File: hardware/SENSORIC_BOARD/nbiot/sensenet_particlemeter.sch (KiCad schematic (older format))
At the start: 102 parts, among them J1 CONN_01X01, J11 CONN_01X01, J13 BARREL_JACK, J18 CONN_01X01, J19 CONN_01X01, J2 CONN_01X01, J21 CONN_01X01, J3 CONN_01X01, J4 CONN_01X01, J5 CONN_01X01, J6 CONN_01X01, P1 SMA_mini, P2 SMA_mini, P3 CONN_02X12, Q1 Q_NMOS_GSD, SW1 SW_DPST, SW2 SW_DIP_x03, SW3 SW_DPST, U1 MC33063, U10 bme280_barebone, U2 stm32f072, U3 QUECTEL_BC95, U4 SIM, U5 CAT24C02, U6 MC33063, U7 M10578-A2, U8 usb_femalee, U9 OLED_128x64

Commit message: snazim se rozchodit novou serii, jebne me z toho z chvili
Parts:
- added C24: 2.2u, SNPM:SMD_0805, symbol C
- added J10, J12, J14, J15, J7, J8, J9: CONN_01X01, SNPM:smd_point_bottom, symbol Conn_01x01
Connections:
- wire segments 392 -> 411
- no-connect marks 87 -> 86
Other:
- note added: "PMEG4010EH,115"
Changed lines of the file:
@@
 	1    0    0    -1
 $EndComp
-NoConn ~ 9750 8800
 NoConn ~ 10050 8800
 NoConn ~ 10150 8800
@@
 	21050 7900 21150 7900
 Wire Wire Line
-	9550 8800 9550 9800
-Wire Wire Line
-	9650 8800 9650 9800
-Wire Wire Line
 	9850 9200 9850 8800
-Wire Wire Line
-	9550 9800 10100 9800
 Wire Wire Line
 	9850 9500 9850 10000
@@
 	1    0    0    -1
 $EndComp
+Wire Wire Line
+	9200 9800 9200 8950
+Wire Wire Line
+	9200 8950 9550 8950
+Wire Wire Line
+	9550 8950 9550 8800
+Wire Wire Line
+	9650 9700 9300 9700
+Wire Wire Line
+	9300 9700 9300 9050
+Wire Wire Line
+	9300 9050 9650 9050
+Wire Wire Line
+	9650 9700 9650 9800
+Wire Wire Line
+	9200 9800 10100 9800
+Wire Wire Line
+	9650 9050 9650 8800
+$Comp
+L C C24
+U 1 1 5BD086E0
+P 9600 9350
+F 0 "C24" H 9625 9450 50  0000 L CNN
+F 1 "2.2u" H 9625 9250 50  0000 L CNN
+F 2 "SNPM:SMD_0805" H 9638 9200 50  0001 C CNN
+F 3 "" H 9600 9350 50  0001 C CNN
+	1    9600 9350
+	1    0    0    -1
+$EndComp
+Wire Wire Line
+	9600 9200 9600 9150
+Wire Wire Line
+	9600 9150 9750 9150
+Wire Wire Line
+	9750 9150 9750 8800
+Wire Wire Line
+	9600 9500 9600 9600
+Wire Wire Line
+	9600 9600 9750 9600
+Wire Wire Line
+	9750 9600 9750 9800
+Connection ~ 9750 9800
+$Comp
+L Conn_01x01 J7
+U 1 1 5BD0A84C
+P 9700 10800
+F 0 "J7" V 9700 10700 50  0000 C CNN
+F 1 "CONN_01X01" V 9800 10800 50  0001 C CNN
+F 2 "SNPM:smd_point_bottom" H 9700 10800 50  0001 C CNN
+F 3 "" H 9700 10800 50  0001 C CNN
+	1    9700 10800
+	0    -1   -1   0
+$EndComp
+$Comp
+L Conn_01x01 J8
+U 1 1 5BD0BD5A
+P 9950 10800
+F 0 "J8" V 9950 10700 50  0000 C CNN
+F 1 "CONN_01X01" V 10050 10800 50  0001 C CNN
+F 2 "SNPM:smd_point_bottom" H 9950 10800 50  0001 C CNN
+F 3 "" H 9950 10800 50  0001 C CNN
+	1    9950 10800
+	0    -1   -1   0
+$EndComp
+$Comp
+L Conn_01x01 J9
+U 1 1 5BD0BEAB
+P 10200 10800
+F 0 "J9" V 10200 10700 50  0000 C CNN
+F 1 "CONN_01X01" V 10300 10800 50  0001 C CNN
+F 2 "SNPM:smd_point_bottom" H 10200 10800 50  0001 C CNN
+F 3 "" H 10200 10800 50  0001 C CNN
+	1    10200 10800
+	0    -1   -1   0
+$EndComp
+$Comp
+L Conn_01x01 J10
+U 1 1 5BD0BFFF
+P 10450 10800
+F 0 "J10" V 10450 10700 50  0000 C CNN
+F 1 "CONN_01X01" V 10550 10800 50  0001 C CNN
+F 2 "SNPM:smd_point_bottom" H 10450 10800 50  0001 C CNN
+F 3 "" H 10450 10800 50  0001 C CNN
+	1    10450 10800
+	0    -1   -1   0
+$EndComp
+$Comp
+L Conn_01x01 J12
+U 1 1 5BD0C156
+P 10700 10800
+F 0 "J12" V 10700 10700 50  0000 C CNN
+F 1 "CONN_01X01" V 10800 10800 50  0001 C CNN
+F 2 "SNPM:smd_point_bottom" H 10700 10800 50  0001 C CNN
+F 3 "" H 10700 10800 50  0001 C CNN
+	1    10700 10800
+	0    -1   -1   0
+$EndComp
+$Comp
+L Conn_01x01 J14
+U 1 1 5BD0C2BC
+P 10950 10800
+F 0 "J14" V 10950 10700 50  0000 C CNN
+F 1 "CONN_01X01" V 11050 10800 50  0001 C CNN
+F 2 "SNPM:smd_point_bottom" H 10950 10800 50  0001 C CNN
+F 3 "" H 10950 10800 50  0001 C CNN
+	1    10950 10800
+	0    -1   -1   0
+$EndComp
+$Comp
+L Conn_01x01 J15
+U 1 1 5BD0C419
+P 11200 10800
+F 0 "J15" V 11200 10700 50  0000 C CNN
+F 1 "CONN_01X01" V 11300 10800 50  0001 C CNN
+F 2 "SNPM:smd_point_bottom" H 11200 10800 50  0001 C CNN
+F 3 "" H 11200 10800 50  0001 C CNN
+	1    11200 10800
+	0    -1   -1   0
+$EndComp
+$Comp
+L GND #PWR093
+U 1 1 5BD0C6C7
+P 11200 11150
+F 0 "#PWR093" H 11200 10900 50  0001 C CNN
+F 1 "GND" H 11200 11000 50  0000 C CNN
+F 2 "" H 11200 11150 50  0001 C CNN
+F 3 "" H 11200 11150 50  0001 C CNN
+	1    11200 11150
+	1    0    0    -1
+$EndComp
+$Comp
+L +5V #PWR094
+U 1 1 5BD0D1A9
+P 10950 11150
+F 0 "#PWR094" H 10950 11000 50  0001 C CNN
+F 1 "+5V" H 10950 11290 50  0000 C CNN
+F 2 "" H 10950 11150 50  0001 C CNN
+F 3 "" H 10950 11150 50  0001 C CNN
+	1    10950 11150
+	-1   0    0    1
+$EndComp
+Text GLabel 10700 11150 3    39   Input ~ 0
+PM_SCK
+Text GLabel 10450 11150 3    39   Input ~ 0
+PM_SDO
+Text GLabel 10200 11150 3    39   Input ~ 0
+OLED_RESET
+Text GLabel 9950 11150 3    39   Input ~ 0
+OLED_D/C
+Text GLabel 9700 11150 3    39   Input ~ 0
+OLED_CS
+Wire Wire Line
+	9700 11000 9700 11150
+Wire Wire Line
+	9950 11000 9950 11150
+Wire Wire Line
+	10200 11000 10200 11150
+Wire Wire Line
+	10450 11000 10450 11150
+Wire Wire Line
+	10700 11000 10700 11150
+Wire Wire Line
+	10950 11000 10950 11150
+Wire Wire Line
+	11200 11000 11200 11150
+Text Notes 14800 1000 0    60   ~ 0
+PMEG4010EH,115
 $EndSCHEMATC

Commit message: zonglovani s repama
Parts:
- C1, C10, C11, C13, C14, C15, C16, C2, C20, C21, C22, C23, C24, C25, C3, C4, C5, C6, C7, C8, C9: symbol C -> sensenet_particlemeter-rescue:C
- C12: value 510pF -> 330pF; symbol C -> sensenet_particlemeter-rescue:C
- C17, C18, C19: symbol CP -> sensenet_particlemeter-rescue:CP
- D1, D11, D3, D5, D6: symbol D_Schottky -> sensenet_particlemeter-rescue:D_Schottky
- D10, D2, D4, D7, D8, D9: symbol LED -> sensenet_particlemeter-rescue:LED
- J1, J10, J11, J12, J14, J15, J18, J19, J2, J21, J3, J4, J5, J6, J7, J8, J9: symbol Conn_01x01 -> sensenet_particlemeter-rescue:Conn_01x01
- J13: symbol Barrel_Jack -> sensenet_particlemeter-rescue:Barrel_Jack
- L1, L2, L3, L5: symbol L -> sensenet_particlemeter-rescue:L
- L4, L6, L7, L8: symbol Ferrite_Bead -> sensenet_particlemeter-rescue:Ferrite_Bead
- LOGO1: symbol LOGO -> sensenet_particlemeter-rescue:LOGO
- P1, P2: symbol SMA_mini -> sensenet_particlemeter-rescue:SMA_mini
- P3: symbol CONN_02X12 -> sensenet_particlemeter-rescue:CONN_02X12
- Q1: symbol Q_NMOS_GSD -> sensenet_particlemeter-rescue:Q_NMOS_GSD
- R1, R10, R11, R12, R13, R14, R17, R18, R19, R2, R20, R22, R23, R24, R25, R26, R27, R28, R29, R3, R4, R5, R6, R7, R8, R9: symbol R -> sensenet_particlemeter-rescue:R
- R15: value 27k -> 2k7; symbol R -> sensenet_particlemeter-rescue:R
- R16: value 10k -> 820R; symbol R -> sensenet_particlemeter-rescue:R
- R21: value tbd -> 100R; symbol R -> sensenet_particlemeter-rescue:R
- SJ16: symbol solder_jumper -> sensenet_particlemeter-rescue:solder_jumper
- SW1, SW3: symbol SW_DPST -> sensenet_particlemeter-rescue:SW_DPST
- SW2: symbol SW_DIP_x03 -> sensenet_particlemeter-rescue:SW_DIP_x03
- U1, U6: symbol MC33063 -> sensenet_particlemeter-rescue:MC33063
- U10: symbol bme280_barebone -> sensenet_particlemeter-rescue:bme280_barebone
- U2: symbol stm32f072 -> sensenet_particlemeter-rescue:stm32f072
- U3: symbol QUECTEL_BC95 -> sensenet_particlemeter-rescue:QUECTEL_BC95
- U4: symbol SIM -> sensenet_particlemeter-rescue:SIM
- U5: symbol CAT24C02 -> sensenet_particlemeter-rescue:CAT24C02
- U7: symbol M10578-A2 -> sensenet_particlemeter-rescue:M10578-A2
- U8: symbol usb_femalee -> sensenet_particlemeter-rescue:usb_femalee
- U9: symbol OLED_128x64 -> sensenet_particlemeter-rescue:OLED_128x64
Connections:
- wire segments 411 -> 498

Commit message: rozdelane upravicky
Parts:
- removed C17: 1000u, SNPM:C_Radial_D10_L16_P5_bottom, symbol sensenet_particlemeter-rescue:CP
- removed J13: BARREL_JACK, SNPM:BARREL_JACK, symbol sensenet_particlemeter-rescue:Barrel_Jack
- added C17: 100n, Capacitor_SMD:C_0805_2012Metric, symbol sensenet_particlemeter-rescue:C
- added C26, C27: 1n, Capacitor_SMD:C_0805_2012Metric, symbol sensenet_particlemeter-rescue:C
- added C28: 22p, Capacitor_SMD:C_0805_2012Metric, symbol sensenet_particlemeter-rescue:C
- added J13: Conn_01x02_Female, Connector_Wire:SolderWirePad_1x02_P3.81mm_Drill1.2mm, symbol Connector:Conn_01x02_Female
- added L9: 39uH, Inductor_SMD:L_Taiyo-Yuden_NR-50xx, symbol sensenet_particlemeter-rescue:L
- added R30: 0R, Resistor_SMD:R_0805_2012Metric, symbol Device:R
- C13: value C -> 100n
- C15: value 1000u -> 470u; footprint SNPM:C_Radial_D10_L16_P5_bottom -> Capacitor_SMD:C_0805_2012Metric
- C18: footprint SNPM:C_Radial_D6.3_L11.2_P2.5_bottom -> Capacitor_THT:CP_Radial_D10.0mm_P5.00mm
- C19: footprint SNPM:C_Radial_D10_L16_P5_bottom -> Capacitor_THT:CP_Radial_D10.0mm_P5.00mm
- L1, L2: value L -> DNP
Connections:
- net labels added: 5V_enable
- net labels removed: batt
- wire segments 498 -> 513
- no-connect marks 86 -> 85
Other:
- moved on the sheet: C15, C19, C25, C7, D1, D3, L4, L7, R12, R13, U4

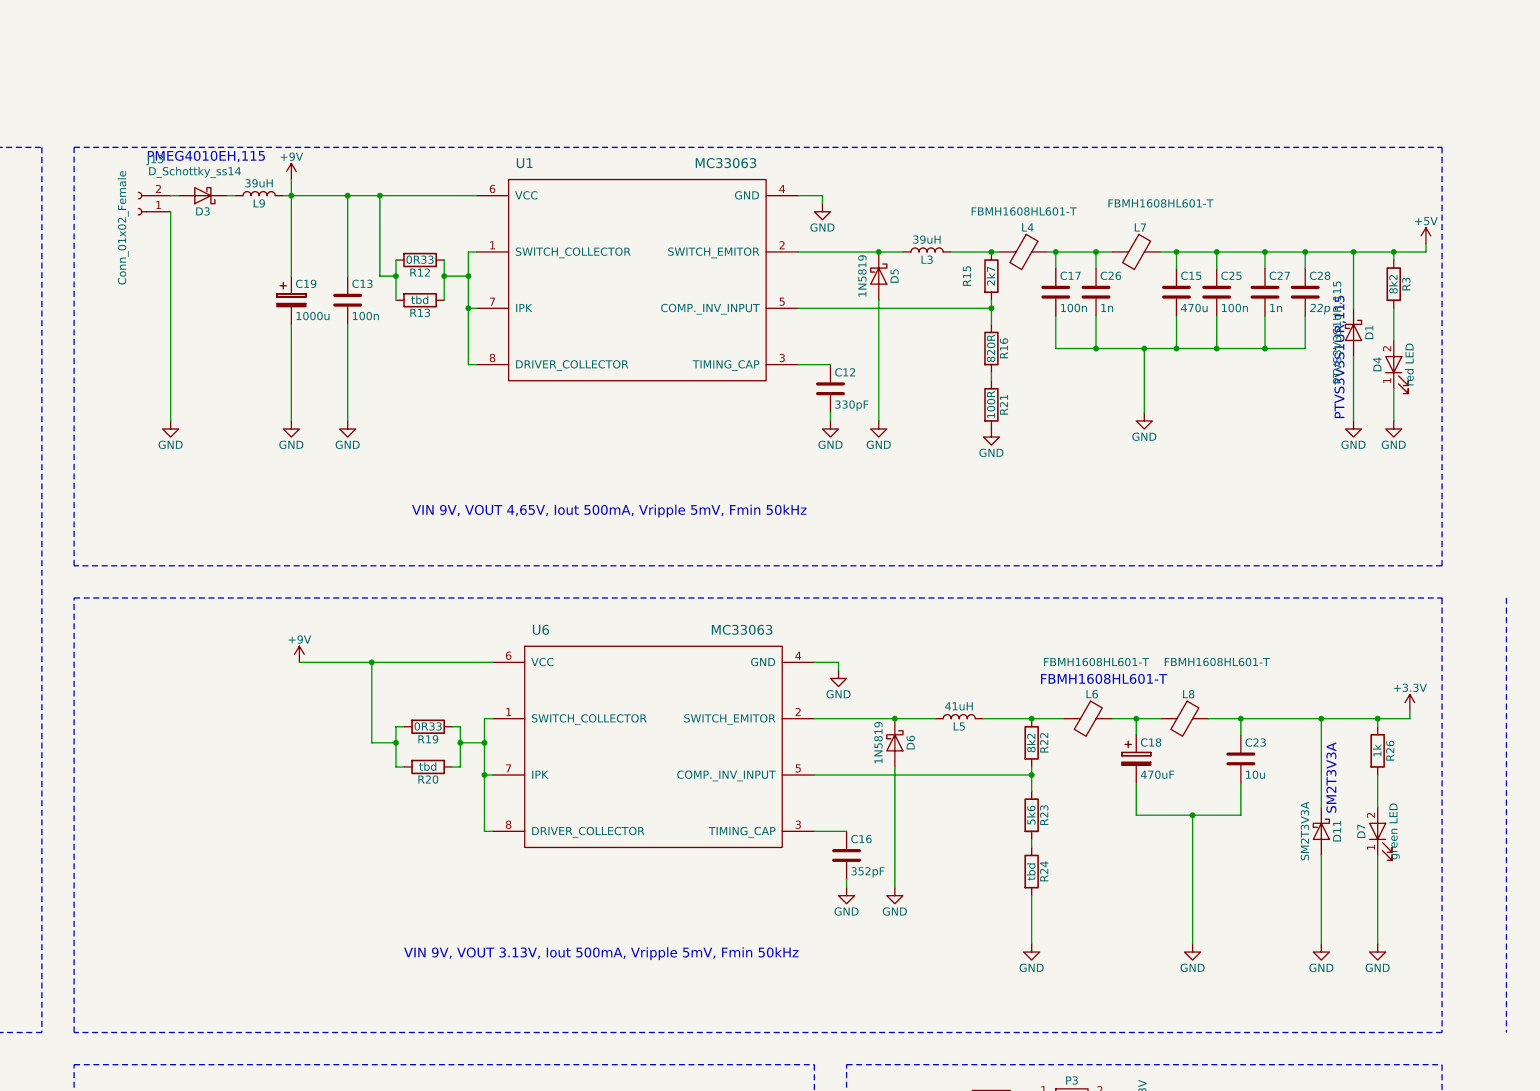
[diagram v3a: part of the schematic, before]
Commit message: V5
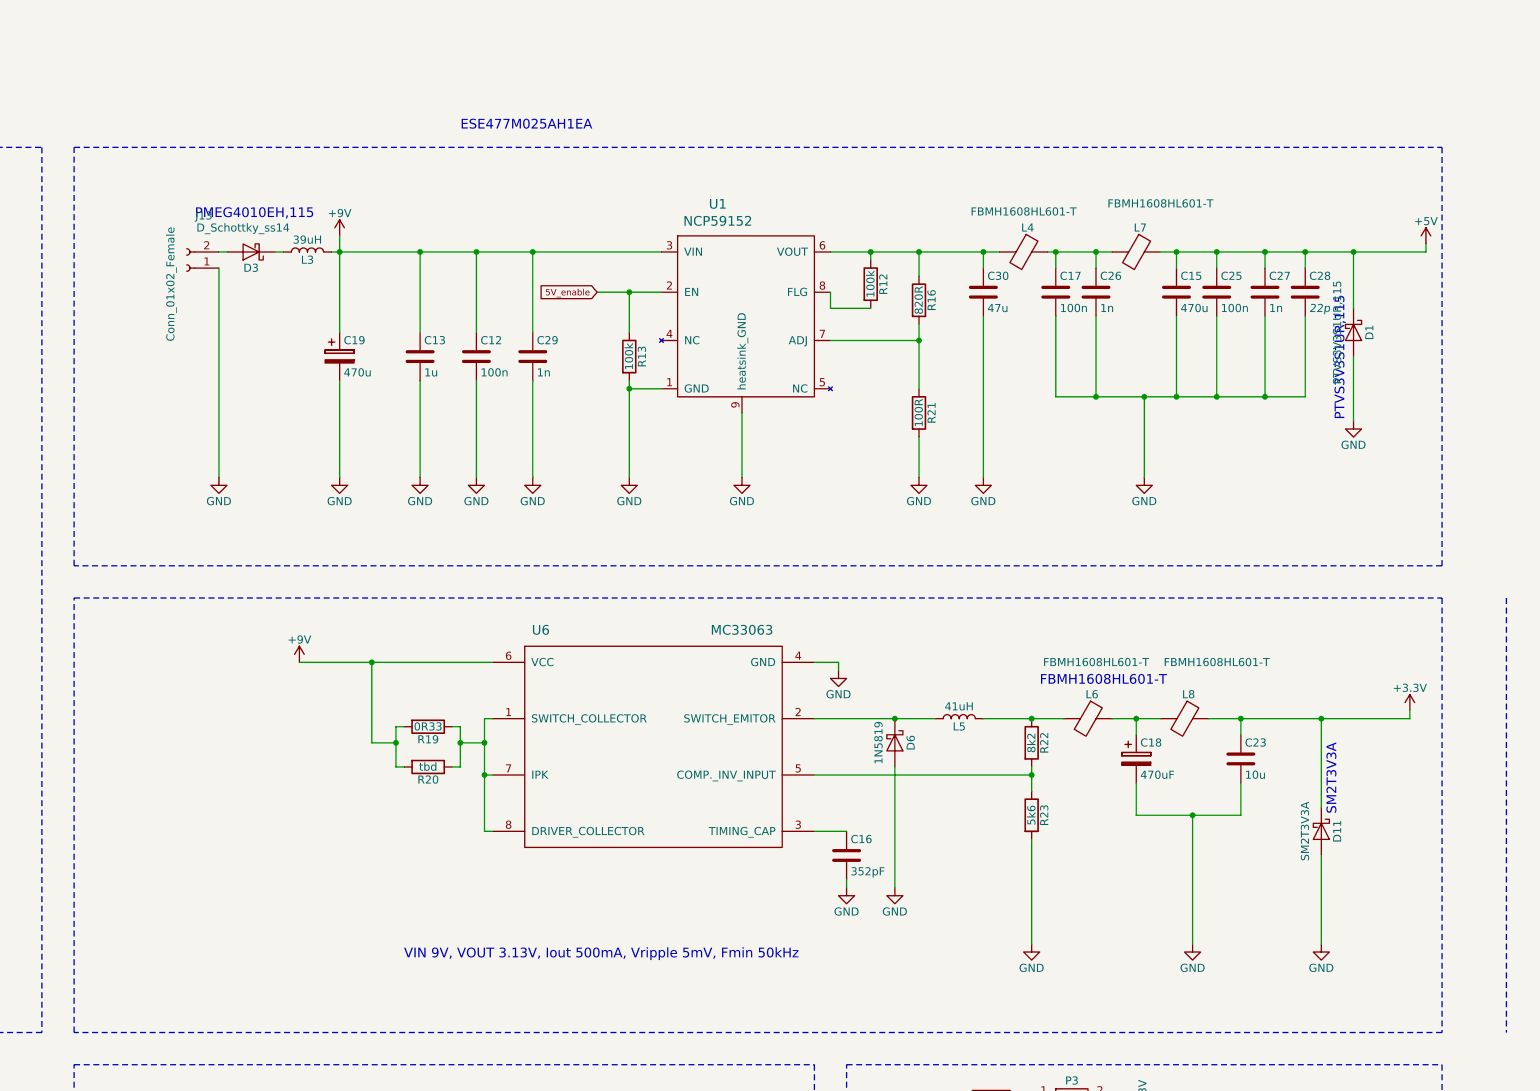
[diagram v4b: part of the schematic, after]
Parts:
- removed D4: red LED, SNPM:SMD_0805_bottom, symbol sensenet_particlemeter-rescue:LED
- removed D5: 1N5819, SNPM:D_SOD-123, symbol sensenet_particlemeter-rescue:D_Schottky
- removed D7: green LED, SNPM:SMD_0805_bottom, symbol sensenet_particlemeter-rescue:LED
- removed L9: 39uH, Inductor_SMD:L_Taiyo-Yuden_NR-50xx, symbol sensenet_particlemeter-rescue:L
- removed R15: 2k7, SNPM:SMD_0805, symbol sensenet_particlemeter-rescue:R
- removed R24: tbd, SNPM:SMD_0805, symbol sensenet_particlemeter-rescue:R
- removed R26: 1k, SNPM:SMD_0805, symbol sensenet_particlemeter-rescue:R
- removed R3: 8k2, SNPM:SMD_0805, symbol sensenet_particlemeter-rescue:R
- removed U1: MC33063, SNPM:SOIC-8_3.9x4.9mm_Pitch1.27mm, symbol sensenet_particlemeter-rescue:MC33063
- added C29: 1n, Capacitor_SMD:C_0805_2012Metric, symbol sensenet_particlemeter-rescue:C
- added C30: 47u, Capacitor_SMD:C_0805_2012Metric, symbol sensenet_particlemeter-rescue:C
- added U1: NCP59152, Package_DFN_QFN:DFN-8-1EP_4x4mm_P0.8mm_EP2.39x2.21mm, symbol NCP59152:NCP59152
- C12: value 330pF -> 100n
- C13: value 100n -> 1u
- C15: footprint Capacitor_SMD:C_0805_2012Metric -> Capacitor_THT:CP_Radial_D10.0mm_P5.00mm
- C19: value 1000u -> 470u
- C25: footprint SNPM:SMD_0805 -> Capacitor_SMD:C_0805_2012Metric
- D1: footprint SNPM:SMD_0805 -> Diode_SMD:D_SOD-123
- R12: value 0R33 -> 100k
- R13: value tbd -> 100k
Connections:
- net +9V: now also C12.1, L3.2, C29.1, U1.3 (VIN); no longer R12.2, R13.2
- net 5V_enable: now also R13.1, U1.2 (EN)
- net GND: now also R13.2, R23.2, C29.2, C30.2, U1.1 (GND), U1.9 (heatsink_GND)
- net at D3.1 (K): now also L3.1
- net at R12.1: now also L4.2, R16.1, C30.1, U1.6 (VOUT); no longer R13.1
- net at R16.2, R21.1: now also U1.7 (ADJ)
- new net: R12.2, U1.8 (FLG)
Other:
- note added: "ESE477M025AH1EA"
- note removed: "VIN 9V, VOUT 4,65V, Iout 500mA, Vripple 5mV, Fmin 50kHz"
- moved on the sheet: C13, C19, D3, J13, L3, R16, R21
